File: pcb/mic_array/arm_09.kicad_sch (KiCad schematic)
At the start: 16 parts, among them U73 IM72D128V01XTMA1, U74 IM72D128V01XTMA1, U75 IM72D128V01XTMA1, U76 IM72D128V01XTMA1, U77 IM72D128V01XTMA1, U78 IM72D128V01XTMA1, U79 IM72D128V01XTMA1, U80 IM72D128V01XTMA1

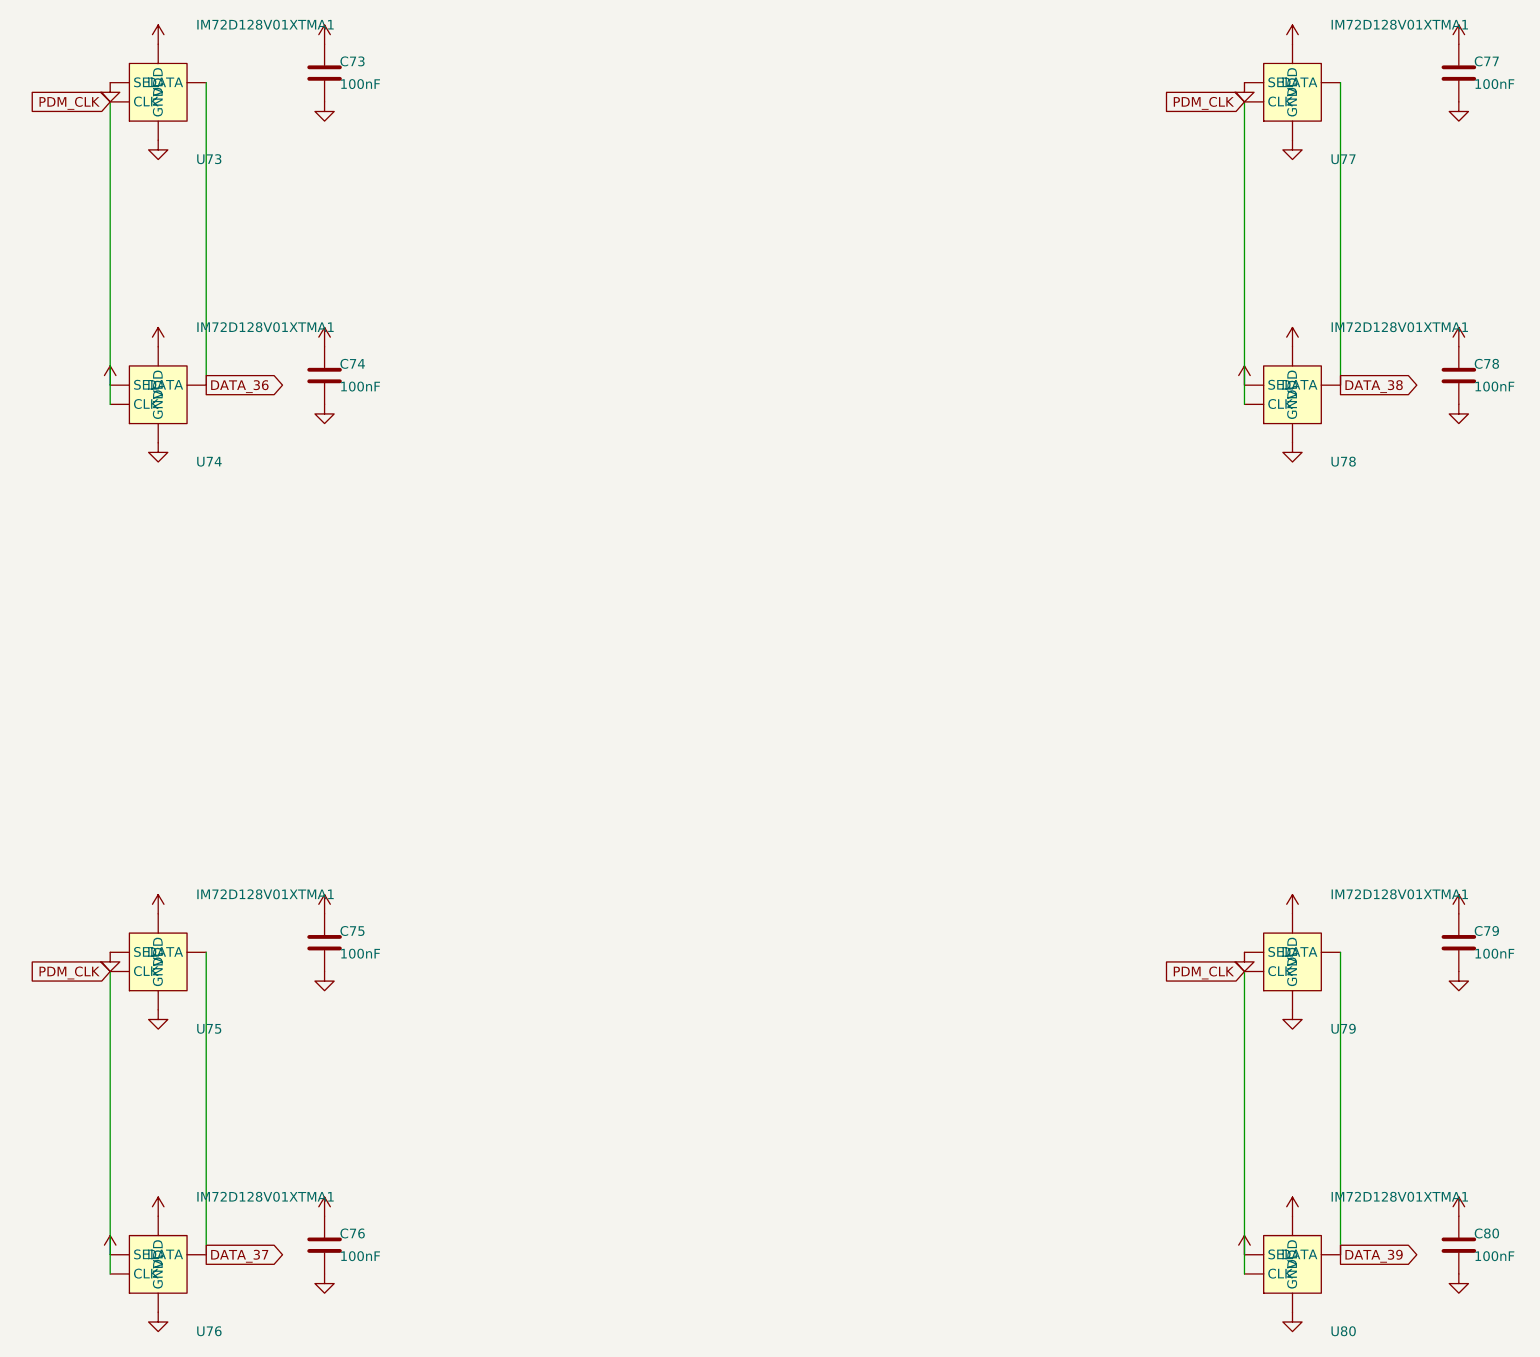
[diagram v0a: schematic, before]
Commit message: Updated.
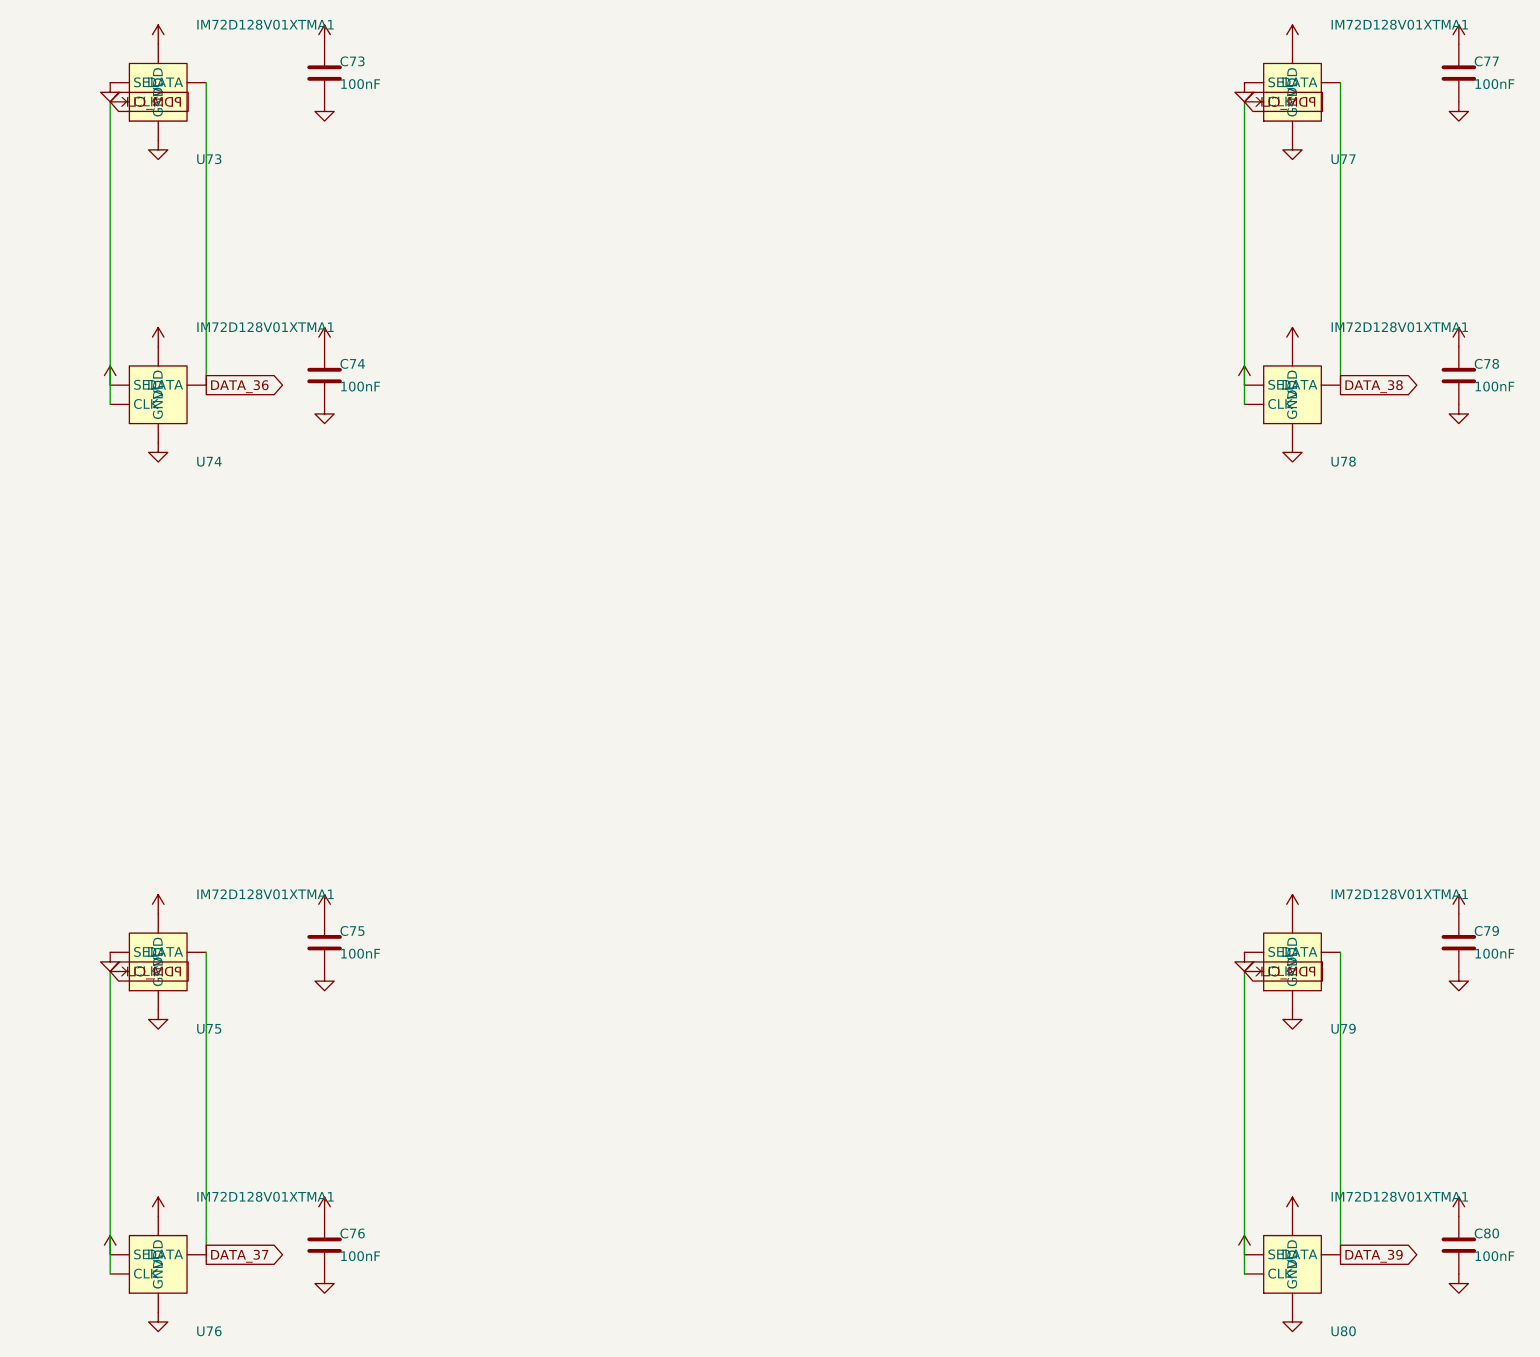
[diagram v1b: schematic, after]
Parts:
- C73, C74, C75, C76, C77, C78, C79, C80: footprint Capacitor_SMD:C_0402_1005Metric -> (none)
- U73, U74, U75, U76, U77, U78, U79, U80: footprint Sensor_Audio:Infineon_PG-LLGA-5-2 -> (none)
